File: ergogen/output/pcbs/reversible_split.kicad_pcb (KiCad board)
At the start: 2 copper layers, 142.6 x 97.7 mm, 19 parts

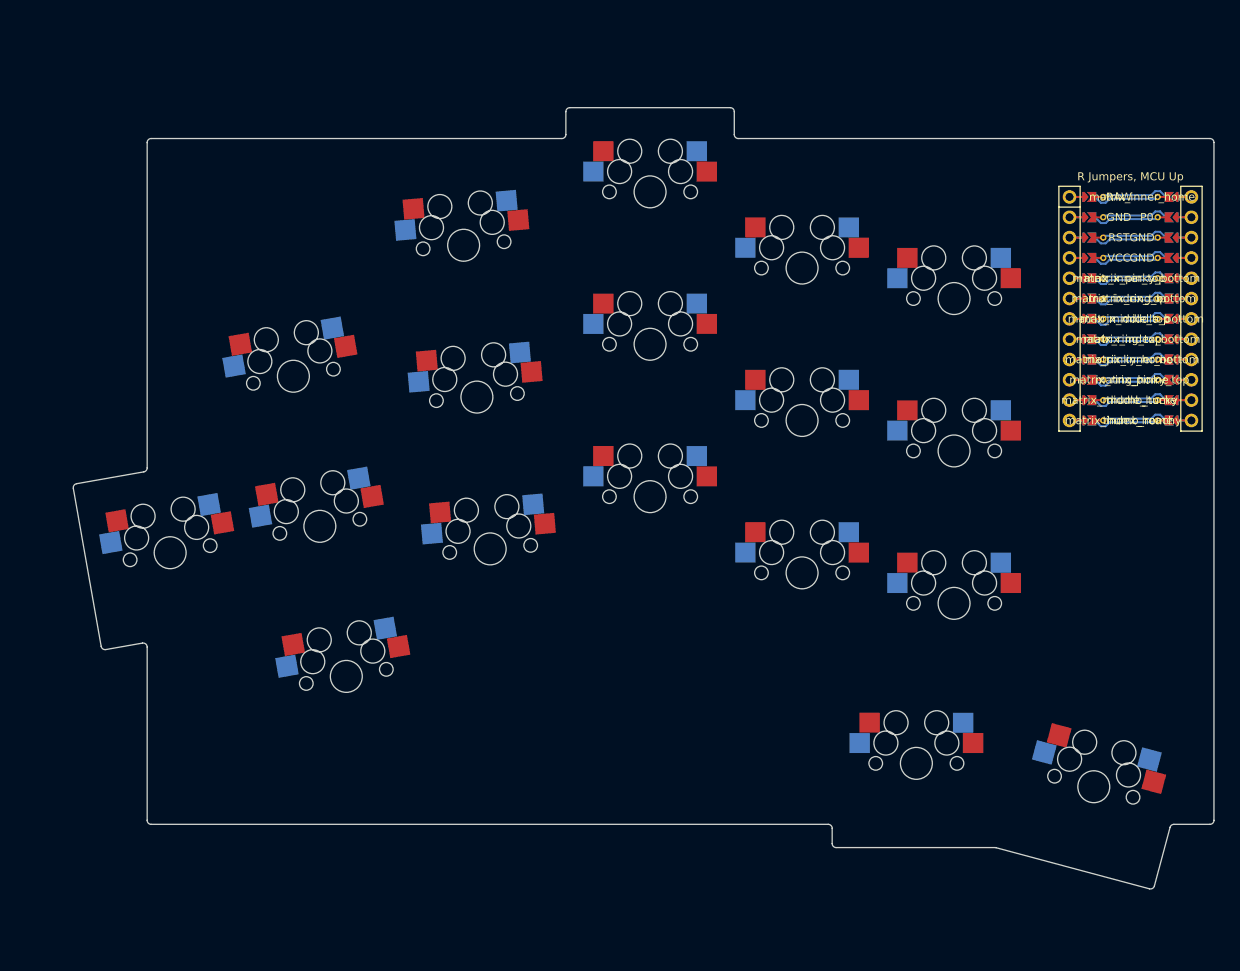
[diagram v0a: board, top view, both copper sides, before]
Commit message: Iteration One (#1)
* Tighter outline

* First complete layout

* Rotated layout experiment

* Updated SMD positions

* First Complete PCB
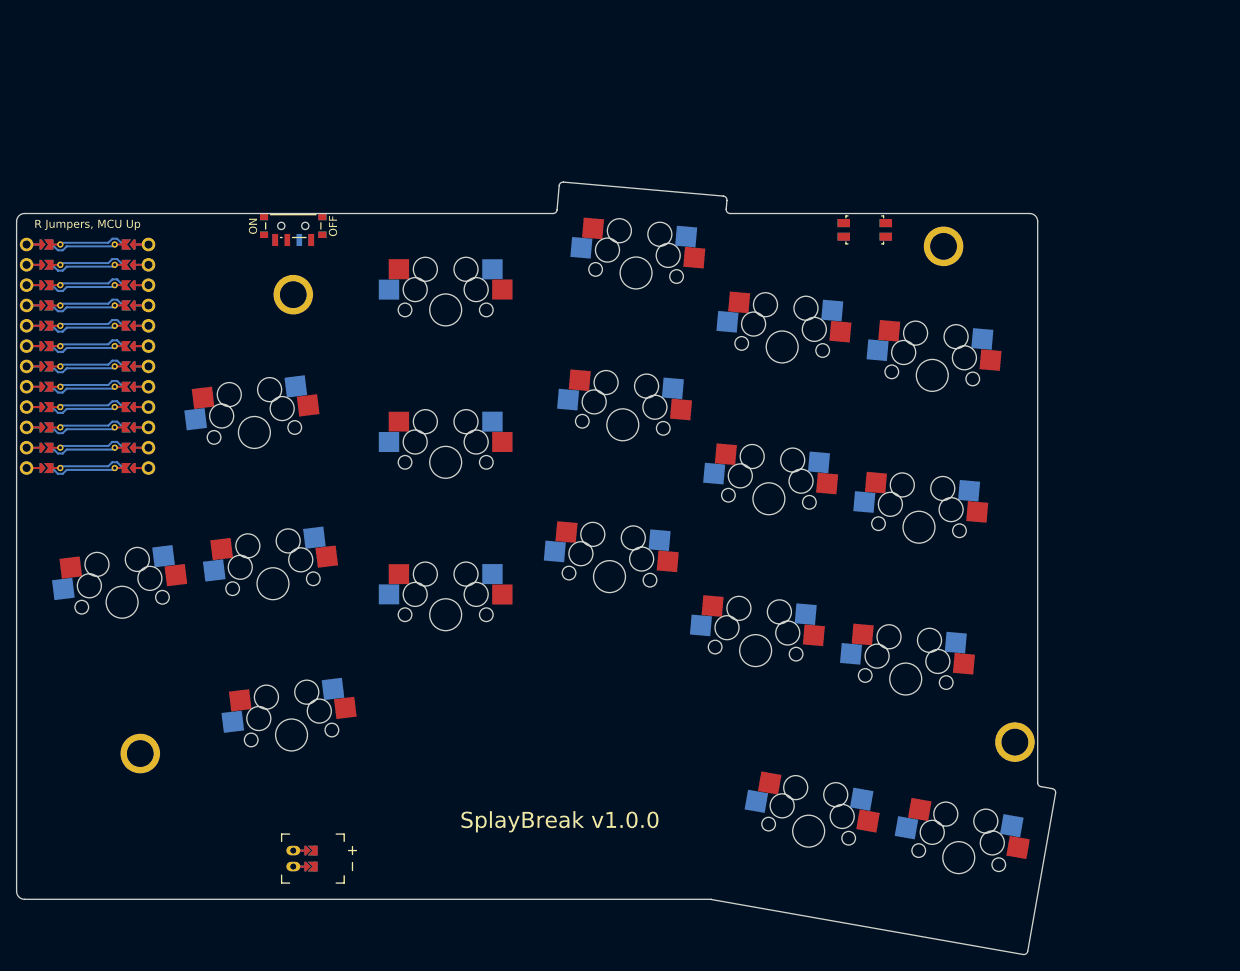
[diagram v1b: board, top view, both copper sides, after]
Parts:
- added H1: , ceoloide:mounting_hole_plated, F.Cu at (136.6, 79.3)
- added H2: , ceoloide:mounting_hole_plated, F.Cu at (117.5, 136.7)
- added H3: , ceoloide:mounting_hole_plated, F.Cu at (226.8, 135.3)
- added H4: , ceoloide:mounting_hole_plated, F.Cu at (217.9, 73.3)
- added JST1: , ceoloide:battery_connector_jst_ph_2, F.Cu at (136.6, 149.8)
- added PWR1: , ceoloide:power_switch_smd_side, F.Cu at (136.6, 70.8)
- added RST1: , ceoloide:reset_switch_smd_side, F.Cu at (208.0, 71.2)
- moved MCU1 130.5 mm to (110.9, 85.8)
- moved S18 19.1 mm to (219.8, 149.7), turned to -10 degrees
- moved S17 15.9 mm to (201.0, 146.4), turned to -10 degrees
- moved S11 11.3 mm to (194.4, 123.8), turned to -5 degrees
- moved S14 11.2 mm to (213.2, 127.4), turned to -5 degrees
- moved S8 11.2 mm to (176.1, 114.6), turned to -5 degrees
- moved S12 10.6 mm to (196.1, 104.9), turned to -5 degrees
- moved S9 10.6 mm to (177.8, 95.6), turned to -5 degrees
- moved S15 10.5 mm to (214.8, 108.4), turned to -5 degrees
- moved S10 10.3 mm to (179.5, 76.6), turned to -5 degrees
- moved S13 10.2 mm to (197.7, 85.9), turned to -5 degrees
- moved S2 10.0 mm to (136.4, 134.4), turned to 7 degrees
- moved S16 9.98 mm to (216.5, 89.4), turned to -5 degrees
- moved S5 9.93 mm to (155.7, 119.3), turned to 0 degrees
- moved S3 9.26 mm to (134.1, 115.5), turned to 7 degrees
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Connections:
- MCU1 pad 101: matrix_inner_home -> matrix_ring_top
- MCU1 pad 102: P0 -> matrix_middle_bottom
- MCU1 pad 105: matrix_pinky_bottom -> matrix_middle_home
- MCU1 pad 106: matrix_ring_bottom -> matrix_middle_top
- MCU1 pad 107: matrix_middle_bottom -> matrix_index_bottom
- MCU1 pad 108: matrix_index_bottom -> matrix_index_home
- MCU1 pad 109: matrix_inner_bottom -> matrix_index_top
- MCU1 pad 110: matrix_pinky_top -> matrix_inner_bottom
- MCU1 pad 111: thumb_tucky -> matrix_inner_home
- MCU1 pad 112: thumb_reachy -> matrix_inner_top
- MCU1 pad 113: matrix_index_home -> thumb_reachy
- MCU1 pad 114: matrix_middle_home -> thumb_tucky
- MCU1 pad 115: matrix_ring_home -> matrix_outer_home
- MCU1 pad 116: matrix_pinky_home -> matrix_pinky_bottom
- MCU1 pad 117: matrix_ring_top -> matrix_pinky_home
- MCU1 pad 118: matrix_middle_top -> matrix_pinky_top
- MCU1 pad 119: matrix_index_top -> matrix_ring_bottom
- MCU1 pad 120: matrix_inner_top -> matrix_ring_home
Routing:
- net JST1_2: track 0.00 -> 3.60 mm
- net JST1_1: track 0.00 -> 3.60 mm
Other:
- board size 142.6 x 97.7 mm -> 129.9 x 96.6 mm
- board text added: "SplayBreak v1.0.0"

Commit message: New ergogen config finalized
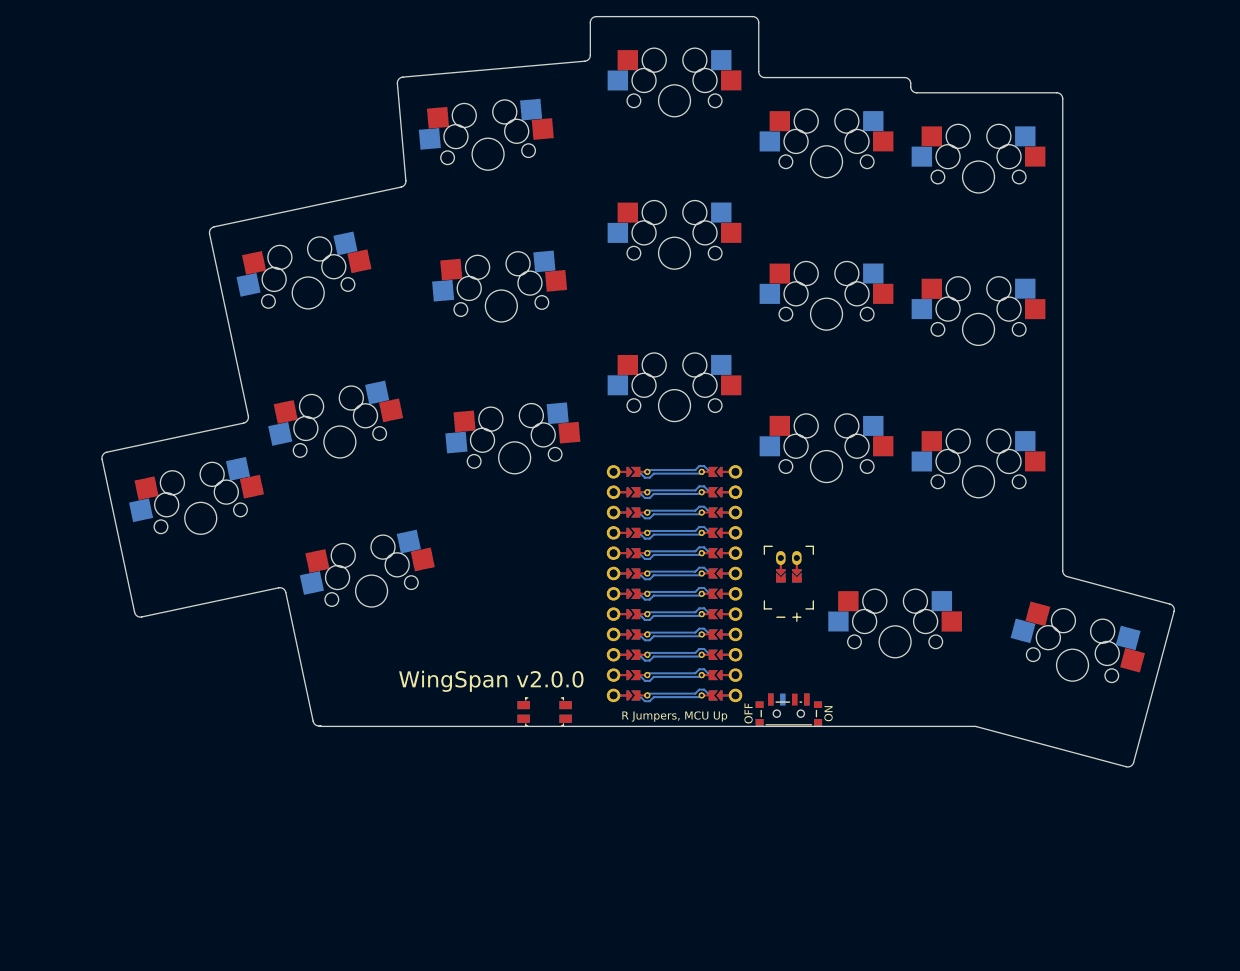
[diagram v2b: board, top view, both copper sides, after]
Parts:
- removed H1, H2, H3, H4: , ceoloide:mounting_hole_plated
- moved PWR1 86.9 mm to (198.6, 131.7), turned to -90 degrees
- moved MCU1 79.6 mm to (184.3, 116.7), turned to 180 degrees
- moved JST1 72.4 mm to (198.6, 112.3), turned to 0 degrees
- moved RST1 72.3 mm to (168.0, 131.5), turned to -180 degrees
- moved S18 27.9 mm to (234.0, 125.7), turned to -15 degrees
- moved S14 26.3 mm to (222.3, 102.7), turned to 0 degrees
- moved S17 26.0 mm to (211.8, 122.7), turned to 0 degrees
- moved S15 25.8 mm to (222.3, 83.7), turned to 0 degrees
- moved S16 25.5 mm to (222.3, 64.6), turned to 0 degrees
- moved S11 24.7 mm to (203.3, 100.8), turned to 0 degrees
- moved S12 24.2 mm to (203.3, 81.8), turned to 0 degrees
- moved S13 23.8 mm to (203.3, 62.7), turned to 0 degrees
- moved S8 22.9 mm to (184.3, 93.2), turned to 0 degrees
- moved S9 22.4 mm to (184.3, 74.2), turned to 0 degrees
- moved S10 22.1 mm to (184.3, 55.1), turned to 0 degrees
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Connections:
- PWR1 pad 2: B+ -> RAW
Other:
- board size 129.9 x 96.6 mm -> 134 x 93.8 mm
- board text added: "WingSpan v2.0.0"
- board text removed: "SplayBreak v1.0.0"
